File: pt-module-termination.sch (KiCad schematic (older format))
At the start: 3 parts

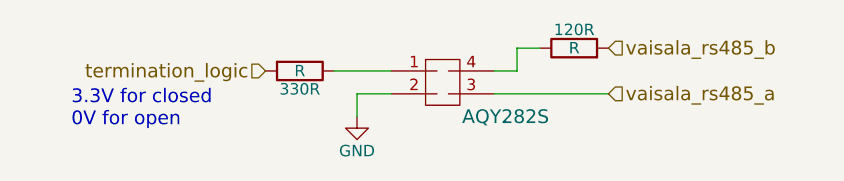
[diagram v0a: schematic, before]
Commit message: Connected EVERYTHING. Ran ERC. There are still some power errors.
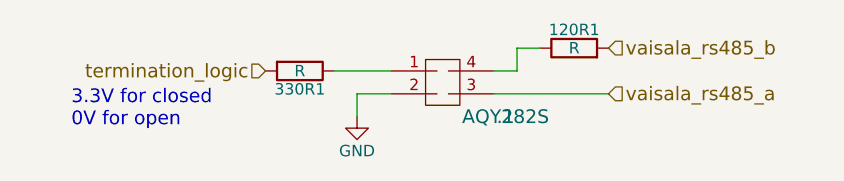
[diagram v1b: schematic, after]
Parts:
- renumbered . to .1, 120R to 120R1, 330R to 330R1
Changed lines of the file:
@@
 LIBS:ftdi
 LIBS:relays
+LIBS:microchip_dspic33dsc
+LIBS:microchip_pic10mcu
+LIBS:microchip_pic12mcu
+LIBS:microchip_pic16mcu
+LIBS:microchip_pic18mcu
+LIBS:microchip_pic24mcu
+LIBS:microchip_pic32mcu
 LIBS:pt-module-cache
 EELAYER 25 0
@@
 vaisala_rs485_b
 $Comp
-L R 120R
+L R 120R1
 U 1 1 5987C0FF
 P 6150 3150
-F 0 "120R" V 6230 3150 50  0000 C CNN
+F 0 "120R1" V 6230 3150 50  0000 C CNN
 F 1 "R" V 6150 3150 50  0000 C CNN
 F 2 "" V 6080 3150 50  0001 C CNN
@@
 termination_logic
 $Comp
-L AQY282S .
+L AQY282S .1
 U 1 1 598B2987
 P 5850 3450
-F 0 "." H 5850 3450 60  0000 C CNN
+F 0 ".1" H 5850 3450 60  0000 C CNN
 F 1 "AQY282S" H 5850 3450 60  0000 C CNN
 F 2 "" H 5850 3450 60  0001 C CNN
@@
 $EndComp
 $Comp
-L GND #PWR?
+L GND #PWR061
 U 1 1 598B2D7C
 P 5200 3450
-F 0 "#PWR?" H 5200 3200 50  0001 C CNN
+F 0 "#PWR061" H 5200 3200 50  0001 C CNN
 F 1 "GND" H 5200 3300 50  0000 C CNN
 F 2 "" H 5200 3450 50  0001 C CNN
@@
 $EndComp
 $Comp
-L R 330R
+L R 330R1
 U 1 1 598B2DEE
 P 4950 3250
-F 0 "330R" V 5030 3250 50  0000 C CNN
+F 0 "330R1" V 5030 3250 50  0000 C CNN
 F 1 "R" V 4950 3250 50  0000 C CNN
 F 2 "" V 4880 3250 50  0001 C CNN
